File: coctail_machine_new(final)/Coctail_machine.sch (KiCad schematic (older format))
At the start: 21 parts, among them M1 Water_pump, M2 Water_pump, M3 Water_punp, SW1 SW, SW2 SW, SW3 SW, SW4 SW_Push, SW5 SW_Push, U1 hx711

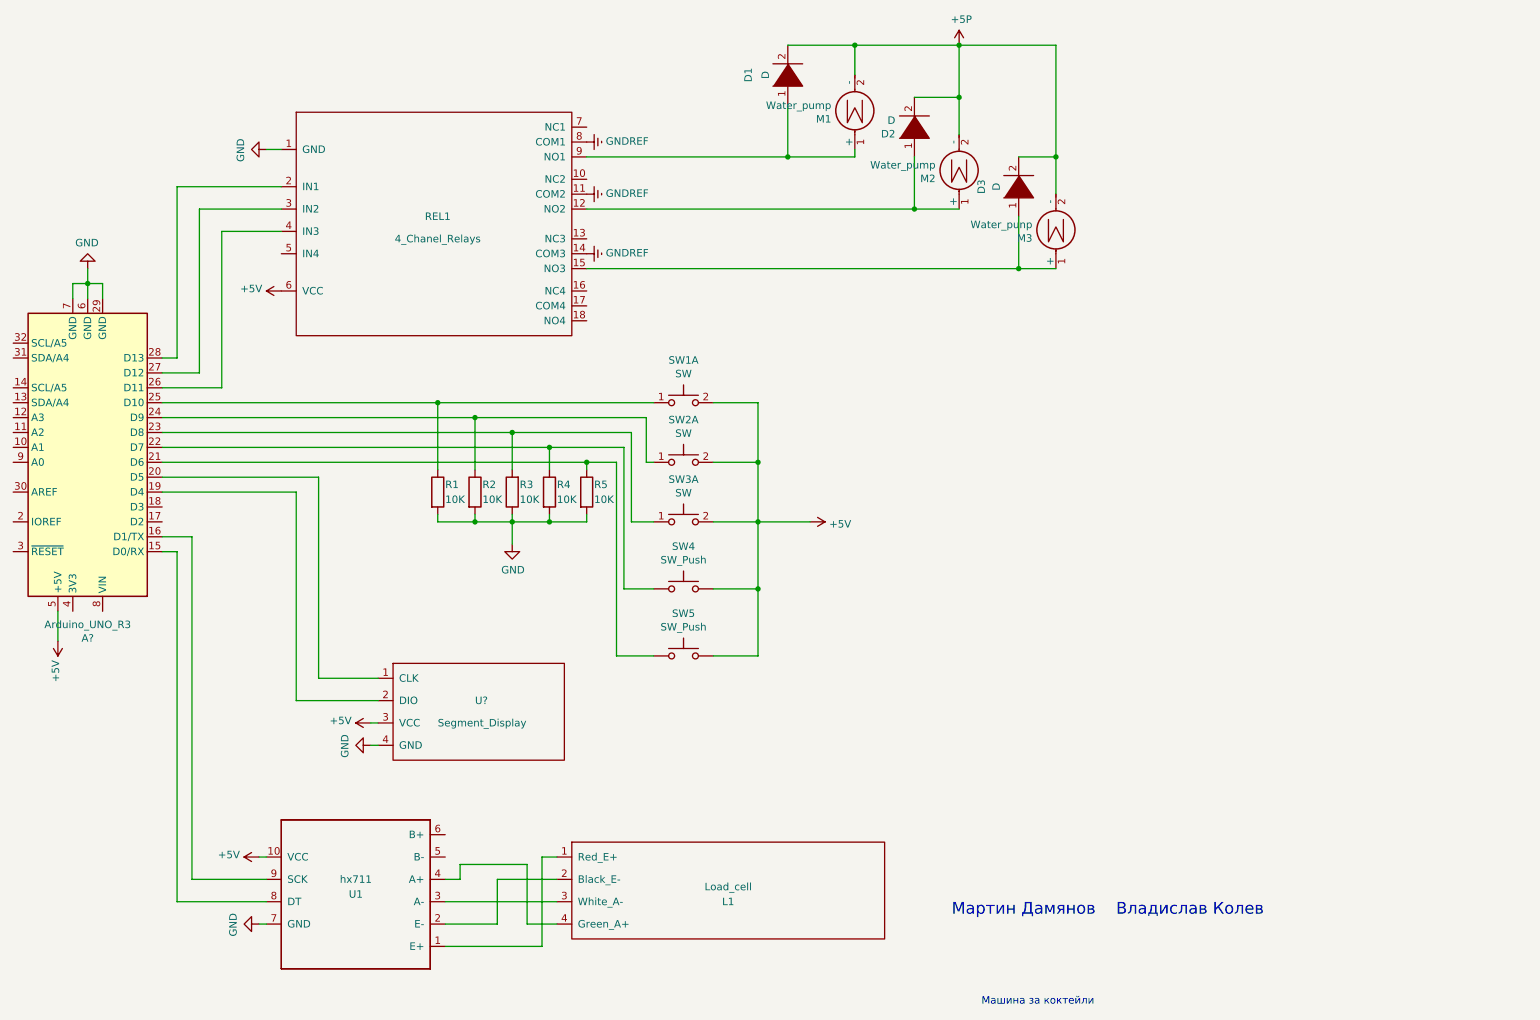
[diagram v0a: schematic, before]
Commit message: scheme update
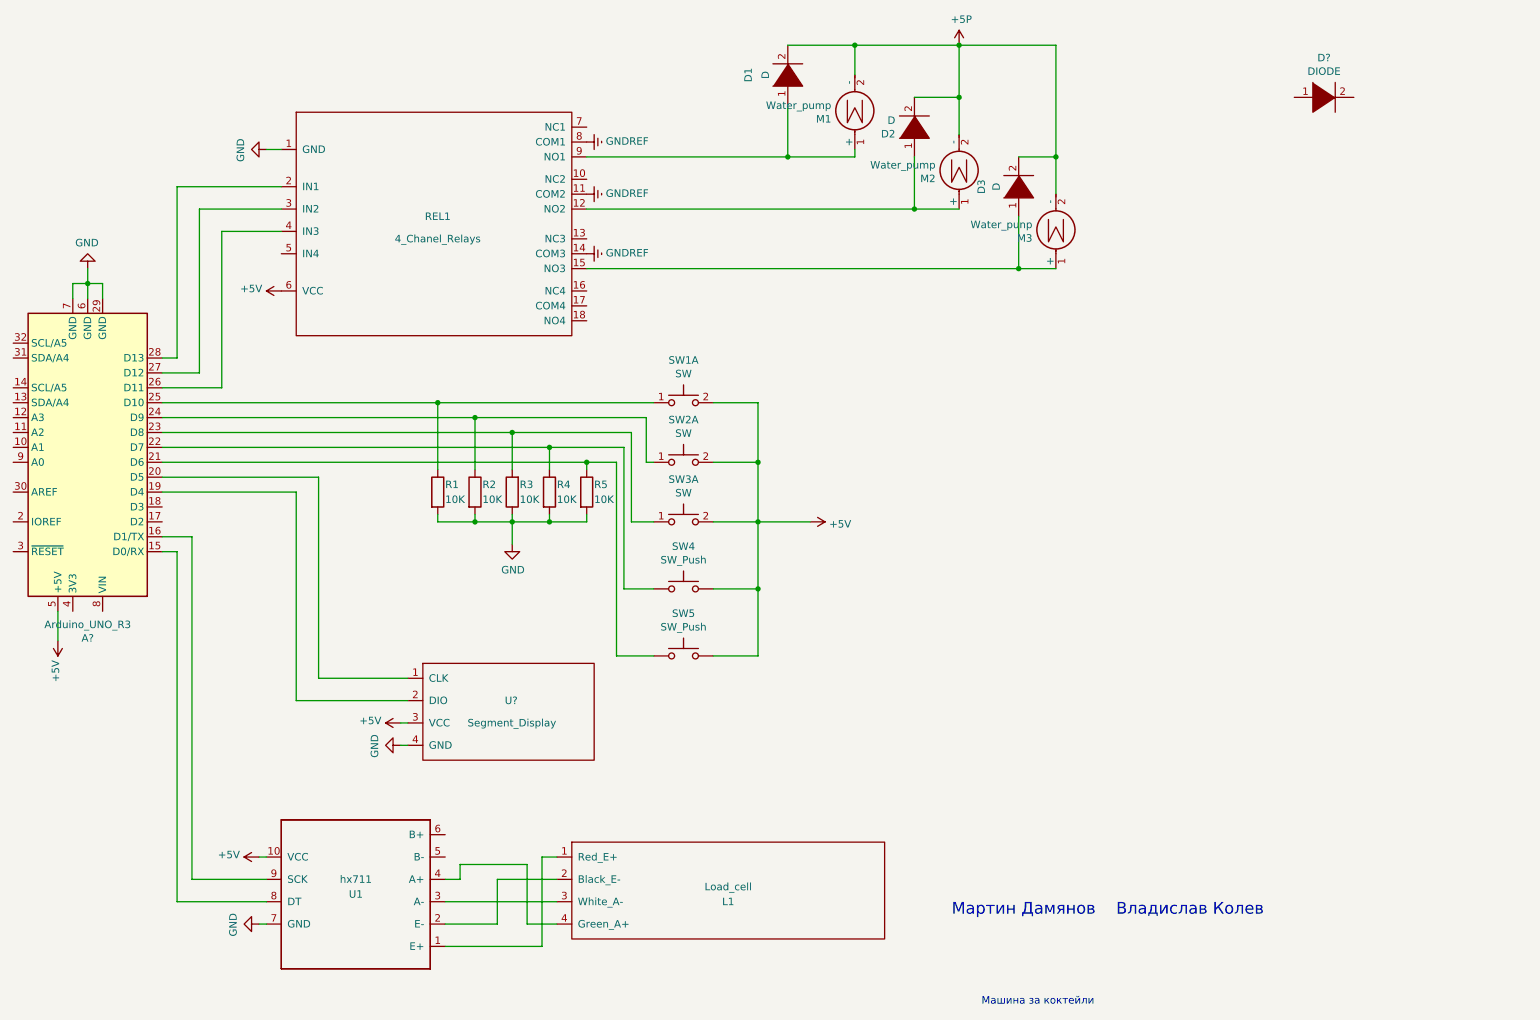
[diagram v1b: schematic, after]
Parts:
- added D?: DIODE, symbol pspice:DIODE
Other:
- moved on the sheet: U?
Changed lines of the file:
@@
 L Arduino:Segment_Display U?
 U 1 1 6037EFCD
-P 4100 5550
-F 0 "U?" H 4000 5650 50  0000 L CNN
-F 1 "Segment_Display" H 3750 5500 50  0000 L CNN
-F 2 "" H 4050 5550 50  0001 C CNN
-F 3 "" H 4050 5550 50  0001 C CNN
-	1    4100 5550
+P 4300 5550
+F 0 "U?" H 4200 5650 50  0000 L CNN
+F 1 "Segment_Display" H 3950 5500 50  0000 L CNN
+F 2 "" H 4250 5550 50  0001 C CNN
+F 3 "" H 4250 5550 50  0001 C CNN
+	1    4300 5550
 	1    0    0    -1
 $EndComp
-Wire Wire Line
-	3350 5300 2950 5300
 Wire Wire Line
 	2950 5300 2950 3950
@@
 Wire Wire Line
 	2800 4050 2800 5450
-Wire Wire Line
-	2800 5450 3350 5450
 Wire Wire Line
 	6550 1050 6550 1250
@@
 L power:+5V #PWR?
 U 1 1 602851FC
-P 3300 5600
-F 0 "#PWR?" H 3300 5450 50  0001 C CNN
-F 1 "+5V" V 3315 5728 50  0000 L CNN
-F 2 "" H 3300 5600 50  0001 C CNN
-F 3 "" H 3300 5600 50  0001 C CNN
-	1    3300 5600
+P 3500 5600
+F 0 "#PWR?" H 3500 5450 50  0001 C CNN
+F 1 "+5V" V 3515 5728 50  0000 L CNN
+F 2 "" H 3500 5600 50  0001 C CNN
+F 3 "" H 3500 5600 50  0001 C CNN
+	1    3500 5600
 	0    -1   -1   0
 $EndComp
 Wire Wire Line
-	3300 5600 3350 5600
+	3500 5600 3550 5600
 Wire Wire Line
 	2550 6950 2600 6950
@@
 L power:GND #PWR?
 U 1 1 6029A263
-P 3300 5750
-F 0 "#PWR?" H 3300 5500 50  0001 C CNN
-F 1 "GND" H 3305 5577 50  0000 C CNN
-F 2 "" H 3300 5750 50  0001 C CNN
-F 3 "" H 3300 5750 50  0001 C CNN
-	1    3300 5750
+P 3500 5750
+F 0 "#PWR?" H 3500 5500 50  0001 C CNN
+F 1 "GND" H 3505 5577 50  0000 C CNN
+F 2 "" H 3500 5750 50  0001 C CNN
+F 3 "" H 3500 5750 50  0001 C CNN
+	1    3500 5750
 	0    1    1    0
 $EndComp
 Wire Wire Line
-	3300 5750 3350 5750
+	3500 5750 3550 5750
+Wire Wire Line
+	2950 5300 3550 5300
+Wire Wire Line
+	2800 5450 3550 5450
+$Comp
+L pspice:DIODE D?
+U 1 1 60309455
+P 9700 1400
+F 0 "D?" H 9700 1665 50  0000 C CNN
+F 1 "DIODE" H 9700 1574 50  0000 C CNN
+F 2 "" H 9700 1400 50  0001 C CNN
+F 3 "~" H 9700 1400 50  0001 C CNN
+	1    9700 1400
+	1    0    0    -1
+$EndComp
 $EndSCHEMATC
